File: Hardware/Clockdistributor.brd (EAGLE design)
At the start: 50 x 50 mm, 50 parts, among them X1 SMA_CONNECTOR, X2 SMA_CONNECTOR, X3 SMA_CONNECTOR, X4 SMA_CONNECTOR, X5 SMA_CONNECTOR, X6 SMA_CONNECTOR, X7 SMA_CONNECTOR, X8 SMA_CONNECTOR

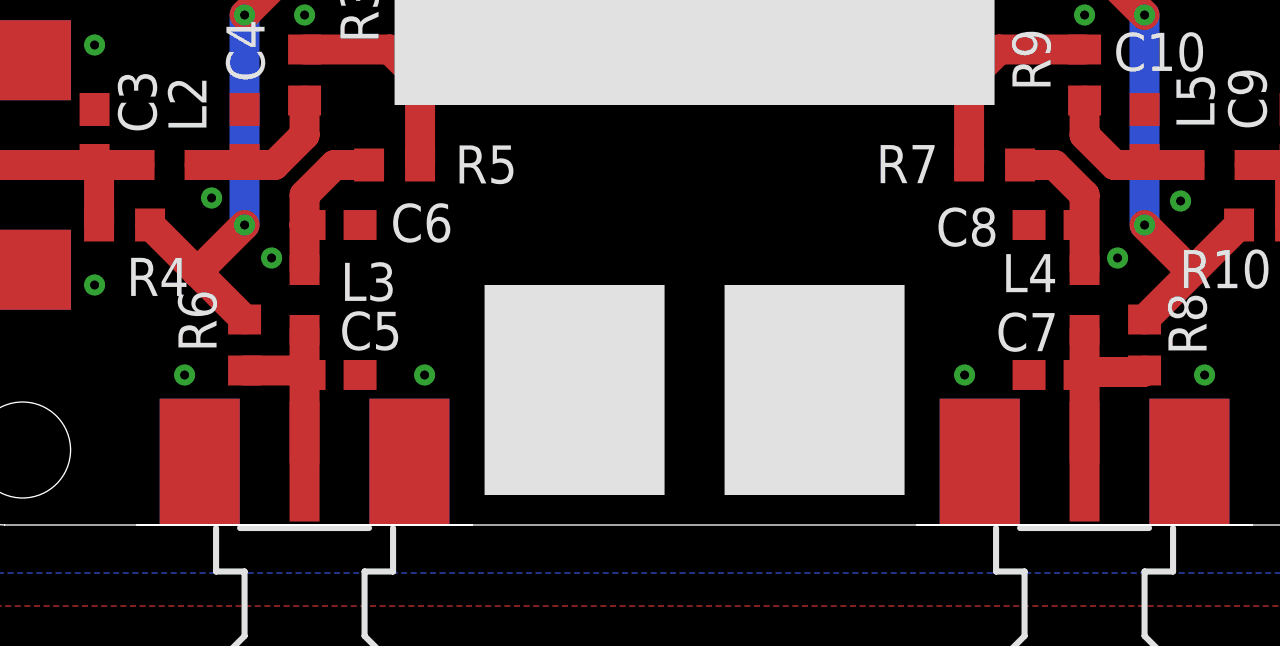
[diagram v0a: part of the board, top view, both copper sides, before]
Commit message: New Gerber files
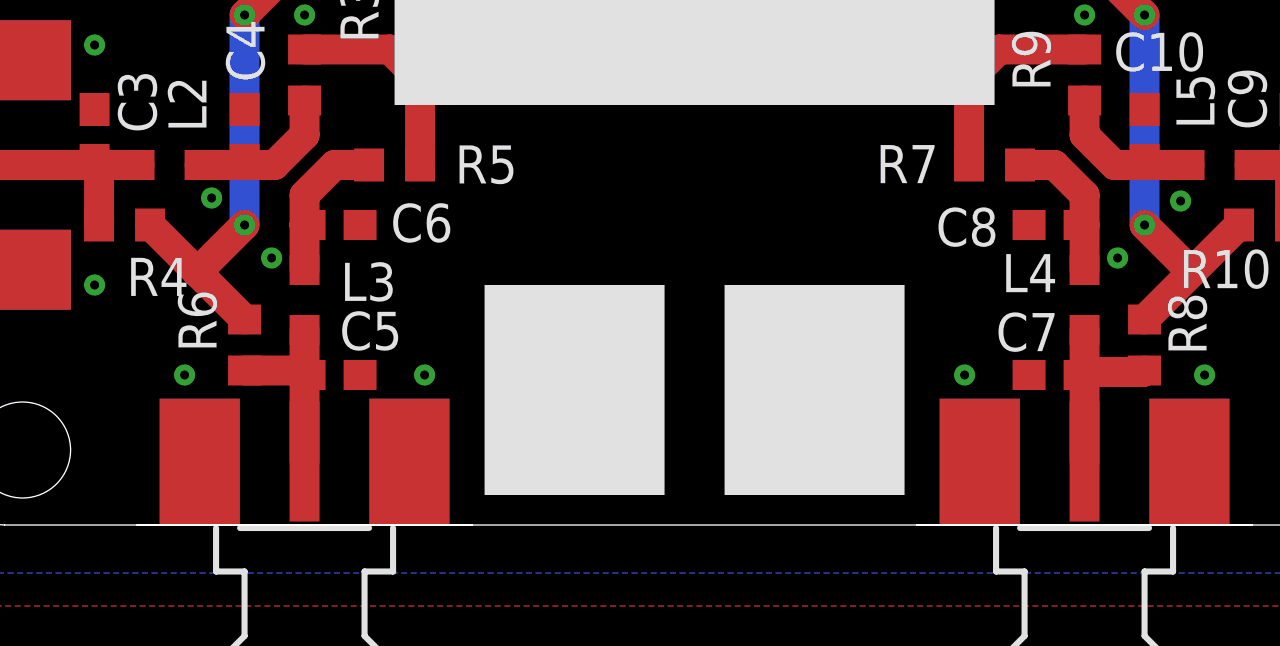
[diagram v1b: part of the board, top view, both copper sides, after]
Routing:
- net GND: track 2.30 -> 4.69 mm
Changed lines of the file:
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@@
 <grid distance="1" unitdist="mm" unit="mm" style="lines" multiple="1" display="yes" altdistance="5" altunitdist="mil" altunit="mil"/>
 <layers>
-<layer number="1" name="Top" color="4" fill="1" visible="no" active="yes"/>
+<layer number="1" name="Top" color="4" fill="1" visible="yes" active="yes"/>
 <layer number="2" name="Route2" color="16" fill="1" visible="no" active="no"/>
 <layer number="3" name="Route3" color="17" fill="1" visible="no" active="no"/>
@@
 <layer number="14" name="Route14" color="22" fill="1" visible="no" active="no"/>
 <layer number="15" name="Route15" color="23" fill="1" visible="no" active="no"/>
-<layer number="16" name="Bottom" color="1" fill="1" visible="no" active="yes"/>
+<layer number="16" name="Bottom" color="1" fill="1" visible="yes" active="yes"/>
 <layer number="17" name="Pads" color="2" fill="1" visible="yes" active="yes"/>
 <layer number="18" name="Vias" color="2" fill="1" visible="yes" active="yes"/>
-<layer number="19" name="Unrouted" color="6" fill="1" visible="no" active="yes"/>
+<layer number="19" name="Unrouted" color="6" fill="1" visible="yes" active="yes"/>
 <layer number="20" name="Dimension" color="24" fill="1" visible="yes" active="yes"/>
 <layer number="21" name="tPlace" color="7" fill="1" visible="yes" active="yes"/>
-<layer number="22" name="bPlace" color="7" fill="1" visible="no" active="yes"/>
-<layer number="23" name="tOrigins" color="15" fill="1" visible="no" active="yes"/>
-<layer number="24" name="bOrigins" color="15" fill="1" visible="no" active="yes"/>
-<layer number="25" name="tNames" color="7" fill="1" visible="yes" active="yes"/>
+<layer number="22" name="bPlace" color="7" fill="1" visible="yes" active="yes"/>
+<layer number="23" name="tOrigins" color="15" fill="1" visible="yes" active="yes"/>
+<layer number="24" name="bOrigins" color="15" fill="1" visible="yes" active="yes"/>
+<layer number="25" name="tNames" color="7" fill="1" visible="no" active="yes"/>
 <layer number="26" name="bNames" color="7" fill="1" visible="no" active="yes"/>
 <layer number="27" name="tValues" color="7" fill="1" visible="no" active="yes"/>
 <layer number="28" name="bValues" color="7" fill="1" visible="no" active="yes"/>
-<layer number="29" name="tStop" color="7" fill="3" visible="yes" active="yes"/>
+<layer number="29" name="tStop" color="7" fill="3" visible="no" active="yes"/>
 <layer number="30" name="bStop" color="7" fill="6" visible="no" active="yes"/>
 <layer number="31" name="tCream" color="7" fill="4" visible="no" active="yes"/>
@@
 <layer number="37" name="tTest" color="7" fill="1" visible="no" active="yes"/>
 <layer number="38" name="bTest" color="7" fill="1" visible="no" active="yes"/>
-<layer number="39" name="tKeepout" color="4" fill="11" visible="no" active="yes"/>
-<layer number="40" name="bKeepout" color="1" fill="11" visible="no" active="yes"/>
-<layer number="41" name="tRestrict" color="4" fill="10" visible="no" active="yes"/>
-<layer number="42" name="bRestrict" color="1" fill="10" visible="no" active="yes"/>
+<layer number="39" name="tKeepout" color="4" fill="11" visible="yes" active="yes"/>
+<layer number="40" name="bKeepout" color="1" fill="11" visible="yes" active="yes"/>
+<layer number="41" name="tRestrict" color="4" fill="10" visible="yes" active="yes"/>
+<layer number="42" name="bRestrict" color="1" fill="10" visible="yes" active="yes"/>
 <layer number="43" name="vRestrict" color="2" fill="10" visible="no" active="yes"/>
 <layer number="44" name="Drills" color="7" fill="1" visible="no" active="yes"/>
 <layer number="45" name="Holes" color="7" fill="1" visible="no" active="yes"/>
-<layer number="46" name="Milling" color="3" fill="1" visible="no" active="yes"/>
+<layer number="46" name="Milling" color="3" fill="1" visible="yes" active="yes"/>
 <layer number="47" name="Measures" color="7" fill="1" visible="no" active="yes"/>
 <layer number="48" name="Document" color="7" fill="1" visible="no" active="yes"/>
 <layer number="49" name="Reference" color="7" fill="1" visible="no" active="yes"/>
 <layer number="51" name="tDocu" color="7" fill="1" visible="yes" active="yes"/>
-<layer number="52" name="bDocu" color="7" fill="1" visible="no" active="yes"/>
+<layer number="52" name="bDocu" color="7" fill="1" visible="yes" active="yes"/>
 <layer number="88" name="SimResults" color="9" fill="1" visible="no" active="no"/>
 <layer number="89" name="SimProbes" color="9" fill="1" visible="no" active="no"/>
@@
 <wire x1="25" y1="25" x2="25" y2="26.15" width="1" layer="1"/>
 <via x="25" y="25" extent="1-16" drill="0.3" shape="octagon"/>
-<wire x1="8.5054" y1="2.1154" x2="8.5054" y2="2.1154" width="0" layer="19" extent="1-16"/>
 <via x="29" y="26" extent="1-16" drill="0.3" shape="octagon"/>
 <via x="31" y="28" extent="1-16" drill="0.3" shape="octagon"/>
@@
 <via x="26" y="25" extent="1-16" drill="0.3" shape="octagon"/>
 <via x="24" y="25" extent="1-16" drill="0.3" shape="octagon"/>
+<wire x1="8.5054" y1="2.1154" x2="8" y2="2.1154" width="0.3048" layer="1"/>
+<wire x1="8" y1="2.1154" x2="8" y2="4" width="0.3048" layer="1"/>
 </signal>
 <signal name="N$2">
@@
 <wire x1="10" y1="5.15" x2="11.95" y2="5.15" width="1" layer="1"/>
 <wire x1="11.95" y1="5.15" x2="12" y2="5.1" width="1" layer="1"/>
-<wire x1="12" y1="5.1" x2="12.15" y2="5" width="0" layer="19" extent="1-1"/>
+<wire x1="12.15" y1="5" x2="12" y2="5" width="0.3048" layer="1"/>
+<wire x1="12" y1="5" x2="12" y2="5.1" width="0.3048" layer="1"/>
 </signal>
 <signal name="N$6">
@@
 <contactref element="R7" pad="1"/>
 <contactref element="C8" pad="1"/>
-<wire x1="38" y1="8.5" x2="38" y2="11" width="1" layer="1"/>
+<wire x1="38" y1="8.5" x2="38" y2="10" width="1" layer="1"/>
+<wire x1="38" y1="10" x2="38" y2="11" width="1" layer="1"/>
 <wire x1="38" y1="11" x2="37" y2="12" width="1" layer="1"/>
 <wire x1="37" y1="12" x2="35.85" y2="12" width="1" layer="1"/>
-<wire x1="38" y1="11" x2="37.85" y2="10" width="0" layer="19" extent="1-1"/>
+<wire x1="37.85" y1="10" x2="38" y2="10" width="0.3048" layer="1"/>
 </signal>
 <signal name="N$9">
@@
 <mfgpreviewcolor name="substratecolor" color="0xFF786E46"/>
 </mfgpreviewcolors>
+<errors>
+</errors>
 </board>
 </drawing>
